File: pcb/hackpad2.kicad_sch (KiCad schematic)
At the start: 30 parts, among them SW1 RotaryEncoder_Switch, SW10 SW_Push, SW11 SW_Push, SW13 SW_Push, SW2 SW_Push, SW3 SW_Push, SW4 SW_Push, SW5 SW_Push, SW6 SW_Push, SW7 SW_Push, U1 MOUDLE-SEEEDUINO-XIAO, U2 ER_OLEDM0.91_1x-I2C

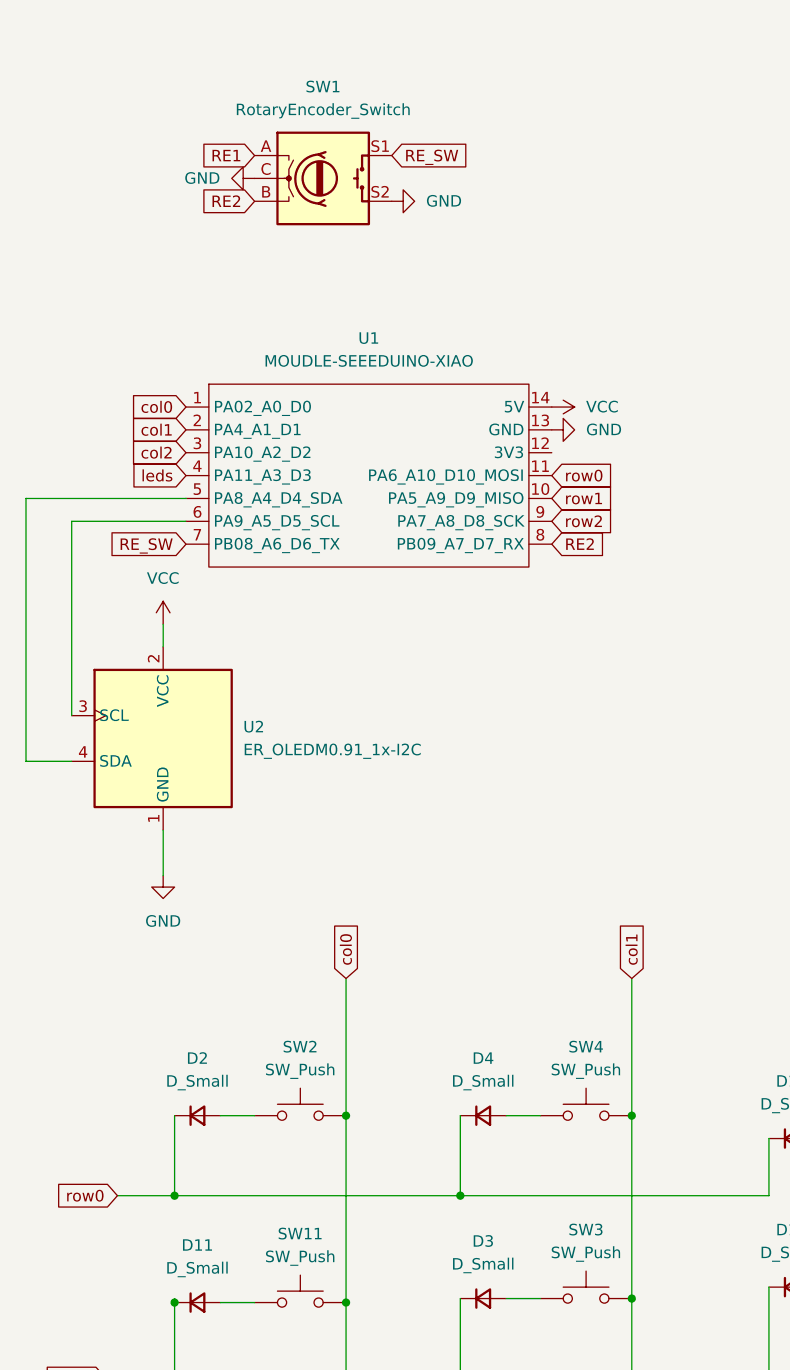
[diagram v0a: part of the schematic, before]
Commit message: ROUTING DONE
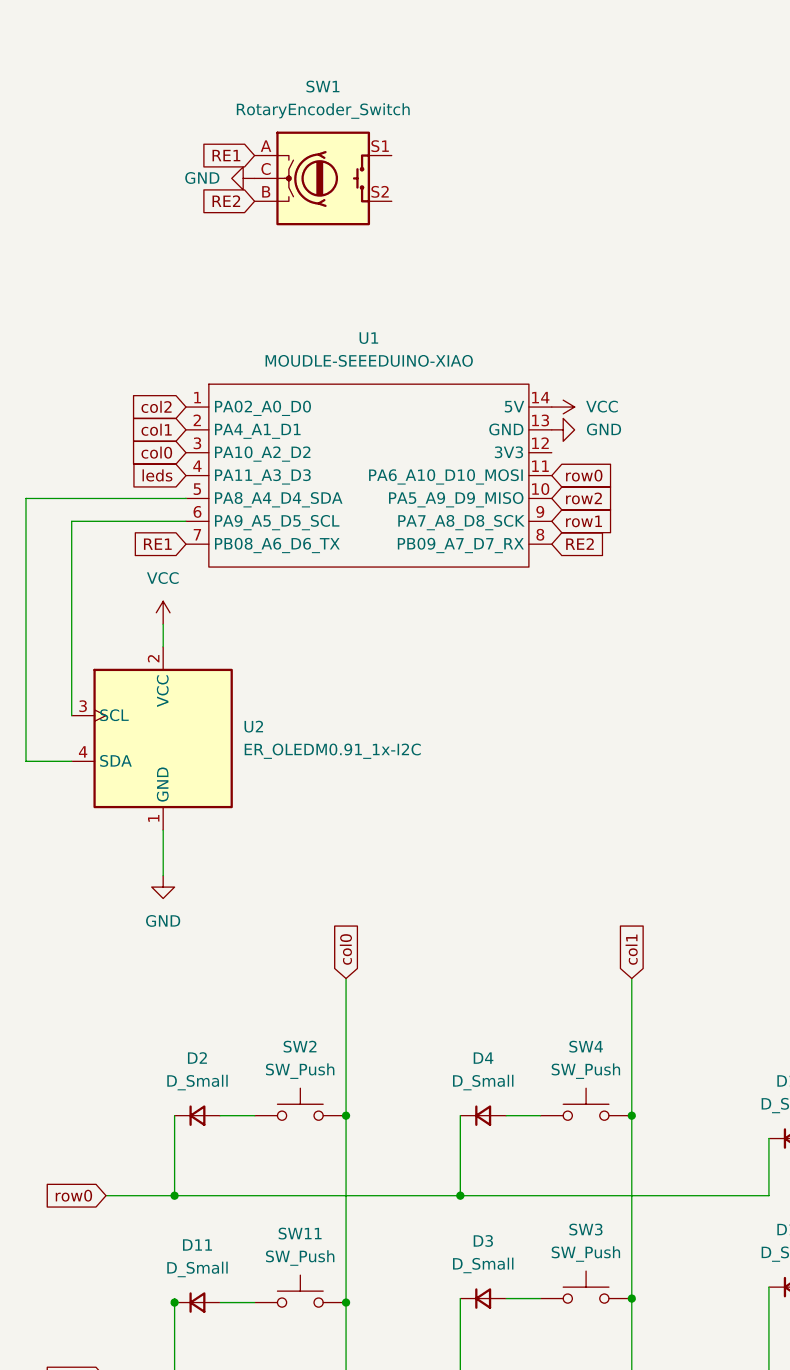
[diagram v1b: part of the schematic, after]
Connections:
- net GND: no longer SW1.S2
- net RE1: now also U1.7 (PB08_A6_D6_TX)
- net col0: now also U1.3 (PA10_A2_D2); no longer U1.1 (PA02_A0_D0)
- net col2: now also U1.1 (PA02_A0_D0); no longer U1.3 (PA10_A2_D2)
- net row1: now also U1.9 (PA7_A8_D8_SCK); no longer U1.10 (PA5_A9_D9_MISO)
- net row2: now also U1.10 (PA5_A9_D9_MISO); no longer U1.9 (PA7_A8_D8_SCK)
- net RE_SW: no longer names the net of SW1.S1
- net RE_SW: no longer U1.7 (PB08_A6_D6_TX)
